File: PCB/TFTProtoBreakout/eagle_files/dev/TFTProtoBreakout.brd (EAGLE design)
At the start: 32.9 x 63.5 mm, 13 parts, among them SW1 PCM12SMTR, SW2 PCM12SMTR, SW3 PCM12SMTR, SW4 PCM12SMTR

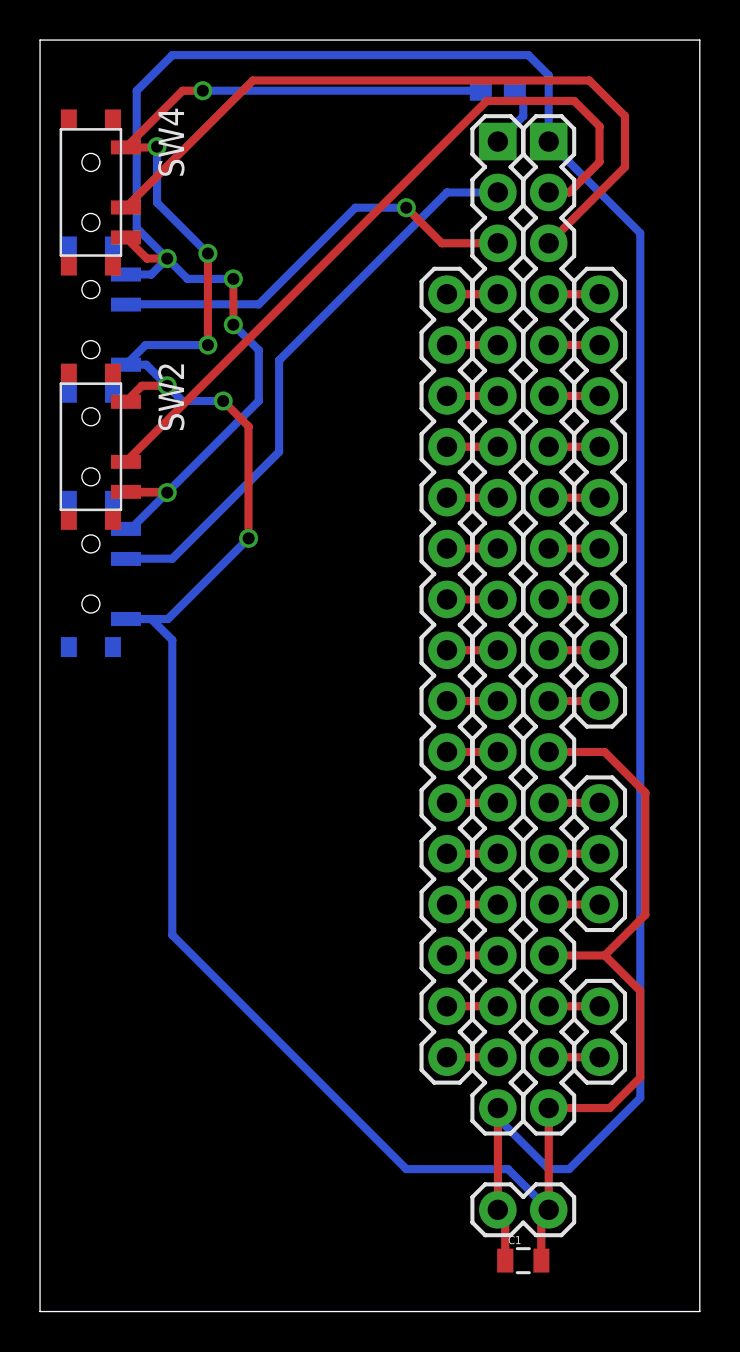
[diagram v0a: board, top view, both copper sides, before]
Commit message: Modified to be a bit more clean.
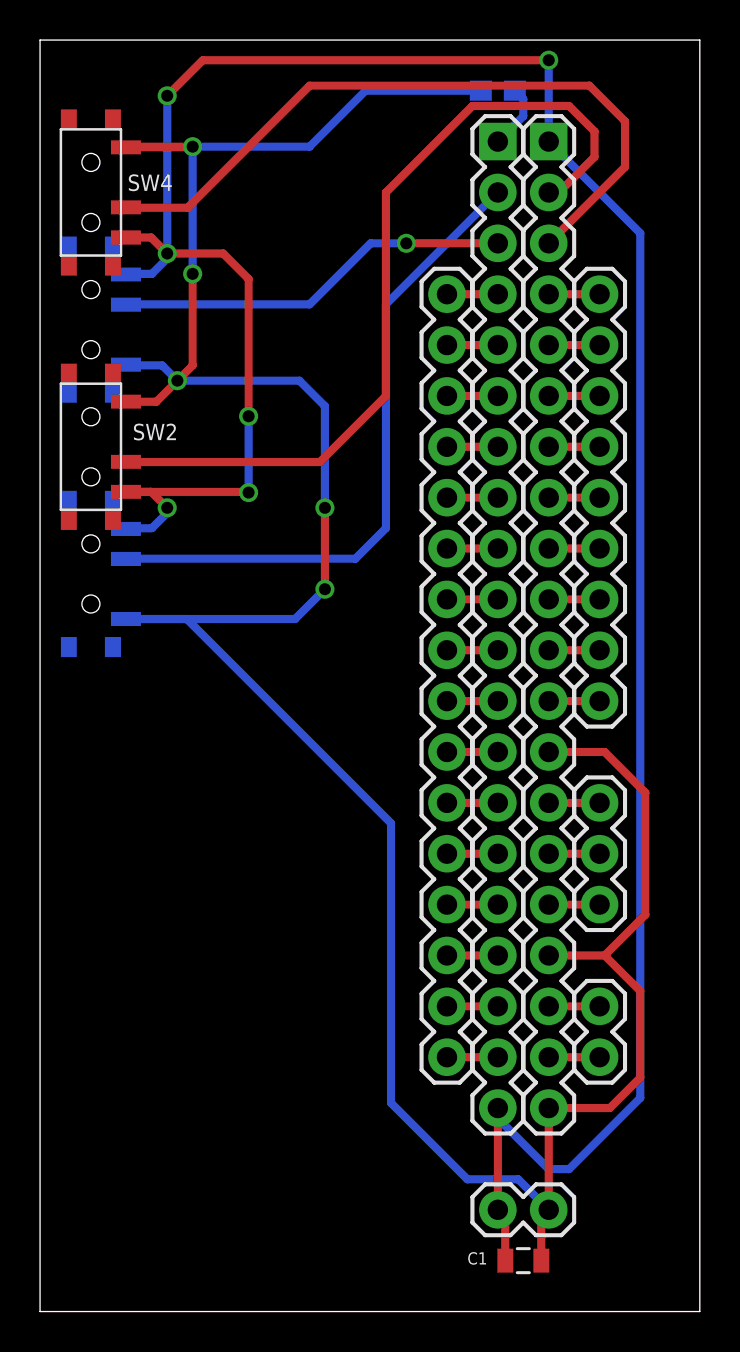
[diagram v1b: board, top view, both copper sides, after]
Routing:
- net GND: track 138.3 -> 146.5 mm, vias 7 -> 5
- net IM1: track 36.6 -> 41.5 mm
- net IM0: track 28.8 -> 32.7 mm
- net IM2: track 21.3 -> 19.8 mm
- net VCC: track 130.3 -> 130.8 mm, vias 4 -> 6
